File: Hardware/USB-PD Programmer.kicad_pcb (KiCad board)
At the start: 2 copper layers, 34 x 34 mm, 36 parts, among them J1 Conn_01x07_Male, J2 Conn_01x04_Male, J3 Conn_01x02_Male, J4 Conn_01x02_Male, J5 Conn_01x02_Male, J6 Conn_01x02_Male, J7 Conn_01x08_Male, SW1 SW_Push, U1 R1501J033B-T1-JE, U2 CH340G/C, Y1 12M

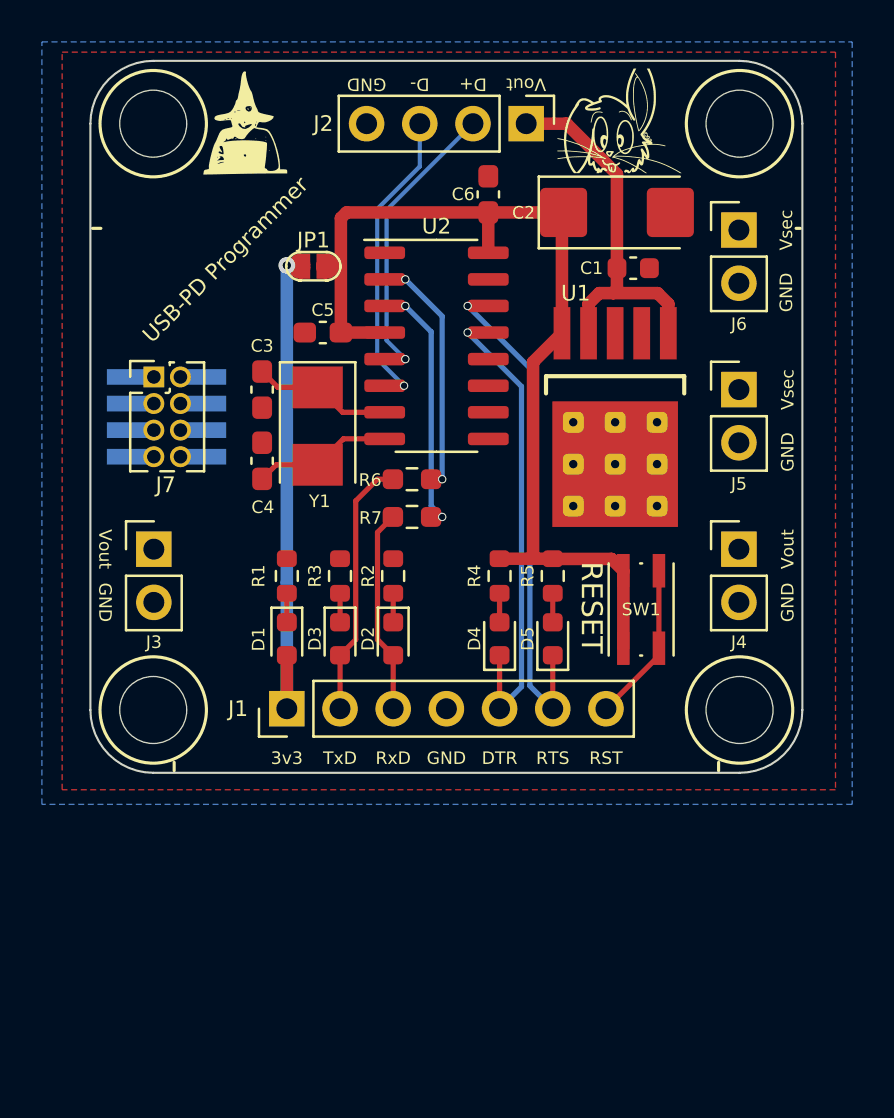
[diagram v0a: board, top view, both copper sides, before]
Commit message: Uber Rework!
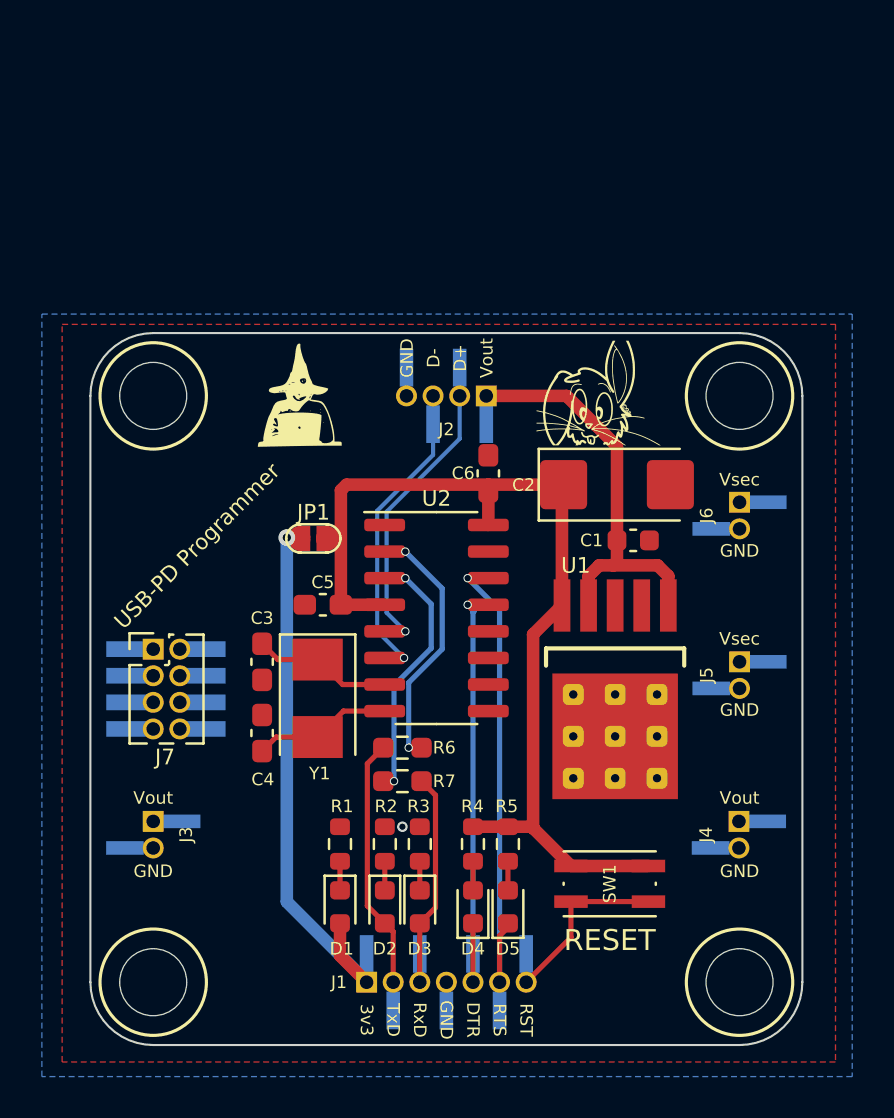
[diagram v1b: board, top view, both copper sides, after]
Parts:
- J1: footprint Connector_PinHeader_2.54mm:PinHeader_1x07_P2.54mm_Vertical -> Tinker:Board_Stacker_7
- J2: footprint Tinker:PinHeader_1x04_P2.54mm_Vertical -> Tinker:Board_Stacker_4
- J3, J4, J5, J6: footprint Tinker:PinHeader_1x02_P2.54mm_Vertical -> Tinker:Board_Stacker_2
- moved J1 13.6 mm to (96.2, 114.0)
- moved C6 13.3 mm to (102.0, 89.7)
- moved G*** 13.3 mm to (93.0, 85.9)
- moved SW1 13.2 mm to (107.8, 109.3), turned to 180 degrees
- moved J2 13.1 mm to (101.9, 86.0)
- moved D1 13.0 mm to (94.9, 110.4)
- moved R1 13.0 mm to (94.9, 107.4)
- moved REF** 13.0 mm to (107.0, 86.5)
- moved J3 13.0 mm to (86.0, 106.3)
- moved J5 13.0 mm to (114.0, 98.7)
- moved J6 13.0 mm to (114.0, 91.1)
- moved J7 13.0 mm to (86.0, 98.1)
- moved C1 13.0 mm to (108.9, 92.9)
- moved C2 13.0 mm to (108.1, 90.2)
- moved C3 13.0 mm to (91.2, 98.7)
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- renumbered D3 to D2, D2 to D3, R3 to R2, R2 to R3
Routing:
- net +3V3: track 23.7 -> 26.2 mm
- net Vout: track 18.1 -> 20.0 mm
- net DTR: track 22.0 -> 20.8 mm
- net Vsec: track 47.3 -> 46.4 mm
- net RST: track 7.64 -> 8.44 mm
- net RTS: track 23.5 -> 22.7 mm
- net GND: vias 0 -> 1
